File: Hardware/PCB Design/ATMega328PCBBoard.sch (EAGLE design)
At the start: 9 parts, among them U1 ATMEGA328P_PDIP

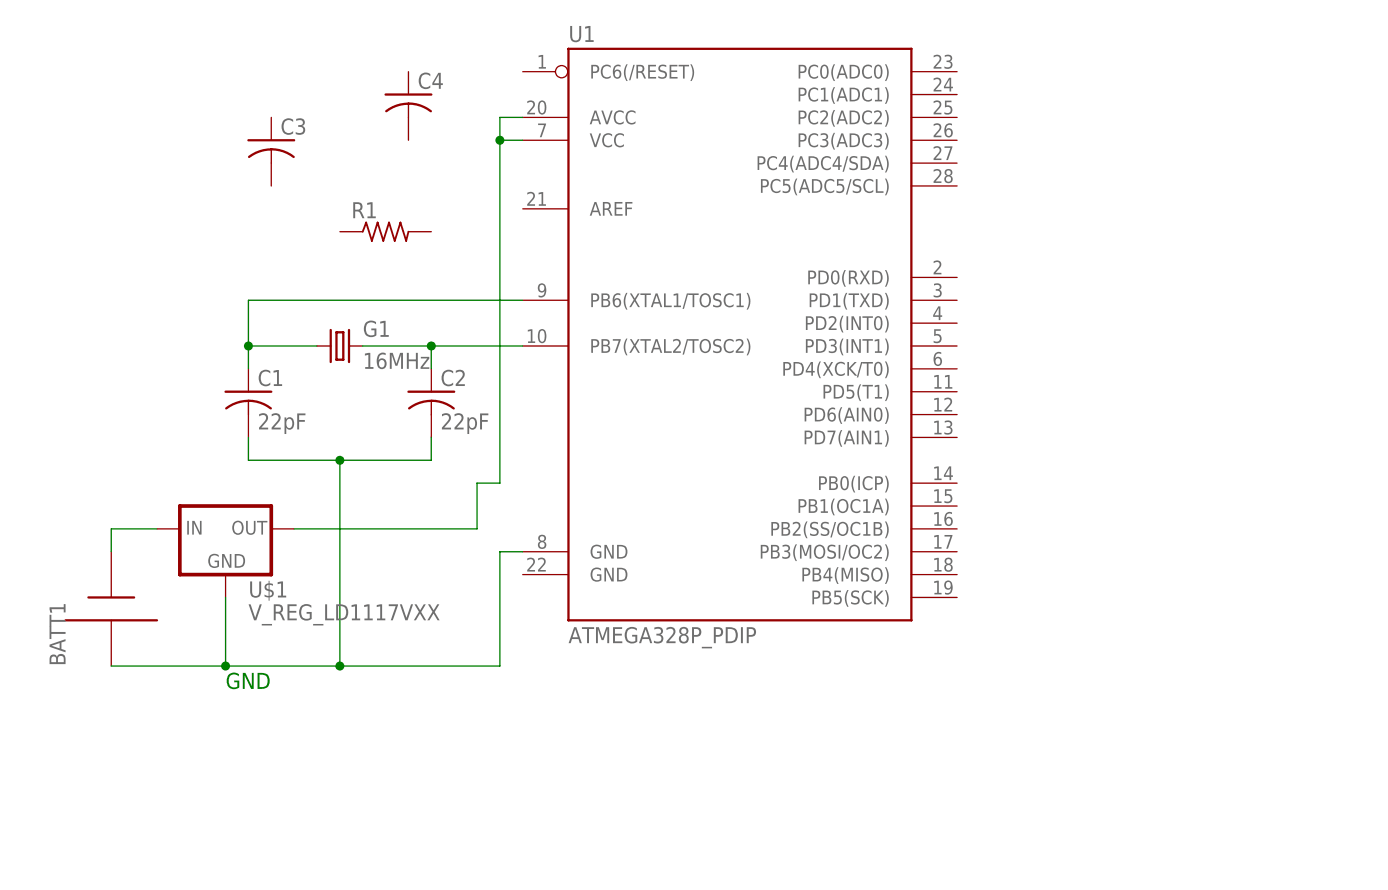
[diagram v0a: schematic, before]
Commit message: finished pcb
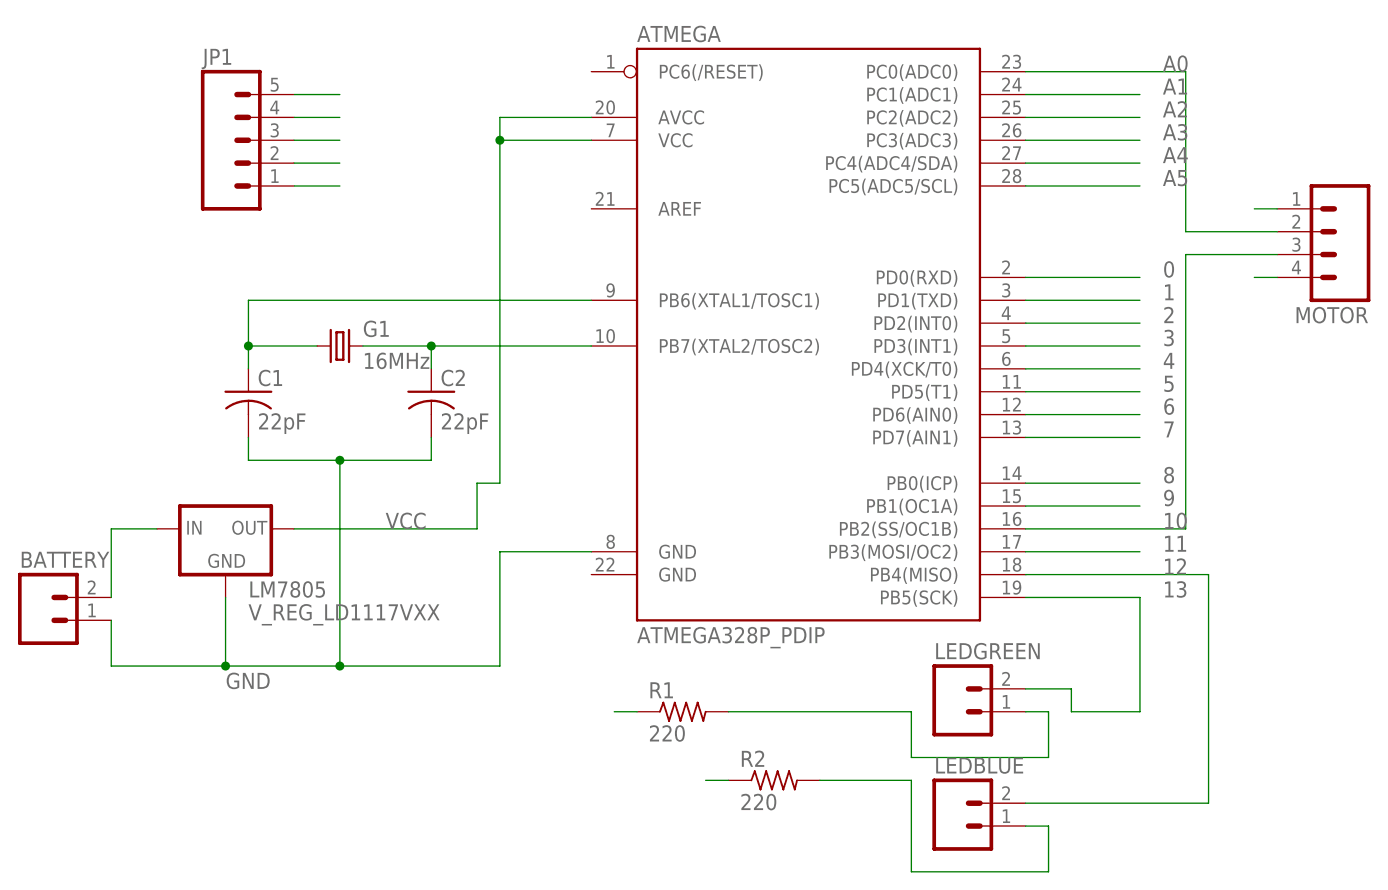
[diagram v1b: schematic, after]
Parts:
- removed BATT1: AAA, adafruit:AAA
- removed C3, C4: (no value), adafruit:C-US050-025X075
- removed U1: ATMEGA328P_PDIP, SparkFun-DigitalIC:ATMEGA328P_PDIP
- added ATMEGA: ATMEGA328P_PDIP, SparkFun-DigitalIC:ATMEGA328P_PDIP
- added BATTERY, LEDBLUE, LEDGREEN: (no value), SparkFun-Connectors:M02JST-PTH-VERT
- added JP1: (no value), SparkFun-Connectors:M05JST-VERT
- added MOTOR: (no value), SparkFun-Connectors:M04JST
- added R2: 220, resistor:R-US_0207/2V
- R1: value (none) -> 220; device resistor:R-US_0207/10 -> resistor:R-US_0207/2V
- renumbered U$1 to LM7805
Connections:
- removed net GND: BATT1.-, C1.2, C2.2, LM7805.GND, U1.GND@1
- new net 0: ATMEGA.PD0(RXD), JP1.4
- new net 1: ATMEGA.PD1(TXD), JP1.3
- new net 10: ATMEGA.PB2(SS/OC1B), MOTOR.3
- new net 11: ATMEGA.PB3(MOSI/OC2)
- new net 12: ATMEGA.PB4(MISO), LEDBLUE.2
- new net 13: ATMEGA.PB5(SCK), LEDGREEN.2
- new net 2: ATMEGA.PD2(INT0)
- new net 3: ATMEGA.PD3(INT1)
- new net 4: ATMEGA.PD4(XCK/T0)
- new net 5: ATMEGA.PD5(T1)
- new net 6: ATMEGA.PD6(AIN0)
- new net 7: ATMEGA.PD7(AIN1), JP1.1
- new net 8: ATMEGA.PB0(ICP)
- new net 9: ATMEGA.PB1(OC1A)
- new net A0: ATMEGA.PC0(ADC0), MOTOR.2
- new net A1: ATMEGA.PC1(ADC1)
- new net A2: ATMEGA.PC2(ADC2)
- new net A3: ATMEGA.PC3(ADC3)
- new net A4: ATMEGA.PC4(ADC4/SDA)
- new net A5: ATMEGA.PC5(ADC5/SCL)
- new net N$3: LEDGREEN.1, R1.2
- new net N$5: LEDBLUE.1, R2.2
- new net N$7: R2.1
- new net VCC: ATMEGA.AVCC, ATMEGA.VCC, JP1.5, LM7805.OUT, MOTOR.1
- new net XBEE2: ATMEGA.GND@1, BATTERY.1, C1.2, C2.2, JP1.2, LM7805.GND, MOTOR.4
- net N$1: now also ATMEGA.PB7(XTAL2/TOSC2); no longer U1.PB7(XTAL2/TOSC2)
- net N$2: now also ATMEGA.PB6(XTAL1/TOSC1); no longer U1.PB6(XTAL1/TOSC1)
- net N$4: now also BATTERY.2; no longer BATT1.+
- net N$6: now also R1.1; no longer LM7805.OUT, U1.AVCC, U1.VCC
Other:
- note added: "0"
- note added: "1"
- note added: "10"
- note added: "11"
- note added: "12"
- note added: "13"
- note added: "2"
- note added: "3"
- note added: "4"
- note added: "5"
- note added: "6"
- note added: "7"
- note added: "8"
- note added: "9"
- note added: "A0"
- note added: "A1"
- note added: "A2"
- note added: "A3"
- note added: "A4"
- note added: "A5"
- note added: "VCC"
- moved on the sheet: R1
